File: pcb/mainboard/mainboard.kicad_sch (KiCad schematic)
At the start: 28 parts, among them J1 Compass, J10 Right, J11 Back, J12 Conn_01x03_Socket, J13 Conn_01x03_Socket, J14 Conn_01x03_Socket, J15 Conn_01x03_Socket, J16 Conn_01x03_Socket, J17 Conn_01x03_Socket, J18 Conn_01x03_Socket, J19 Conn_01x03_Socket, J2 ESP, J20 Conn_01x03_Socket, J21 Conn_01x03_Socket, J22 Conn_01x03_Socket, J23 Conn_01x03_Socket, J24 Conn_01x03_Socket, J25 Conn_01x03_Socket, J26 Conn_01x03_Socket, J3 ESP_, J4 OLED, J5 MUX_, J6 MUX, J7 Drive, J8 CAM, J9 Left, SW1 Start, SW2 Set

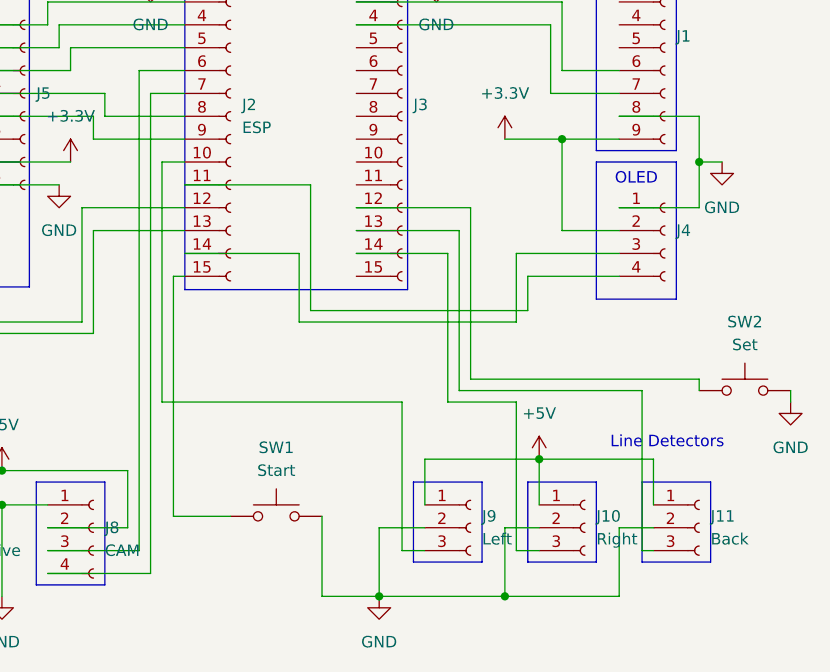
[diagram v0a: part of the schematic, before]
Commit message: IR ring
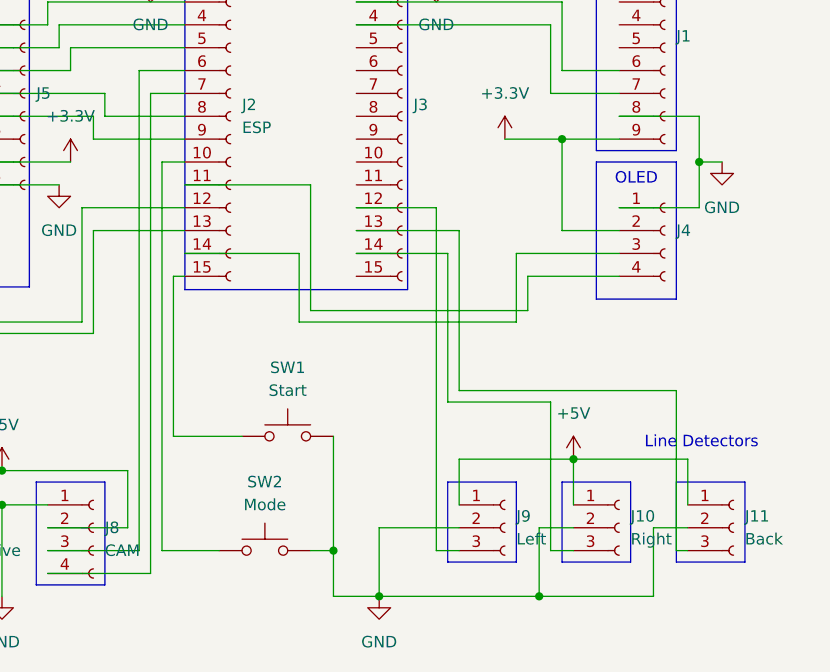
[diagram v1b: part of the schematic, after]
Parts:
- SW2: value Set -> Mode
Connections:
- net at J9.3 (Pin_3): now also J3.12 (Pin_12); no longer J2.10 (Pin_10)
- net at SW2.1: now also J2.10 (Pin_10); no longer J3.12 (Pin_12)
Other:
- moved on the sheet: J10, J11, J9, SW1, SW2
